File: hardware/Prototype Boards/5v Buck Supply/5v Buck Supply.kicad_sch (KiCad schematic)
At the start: 3 parts, among them J1 BATT, U1 INA180A1IDBVT

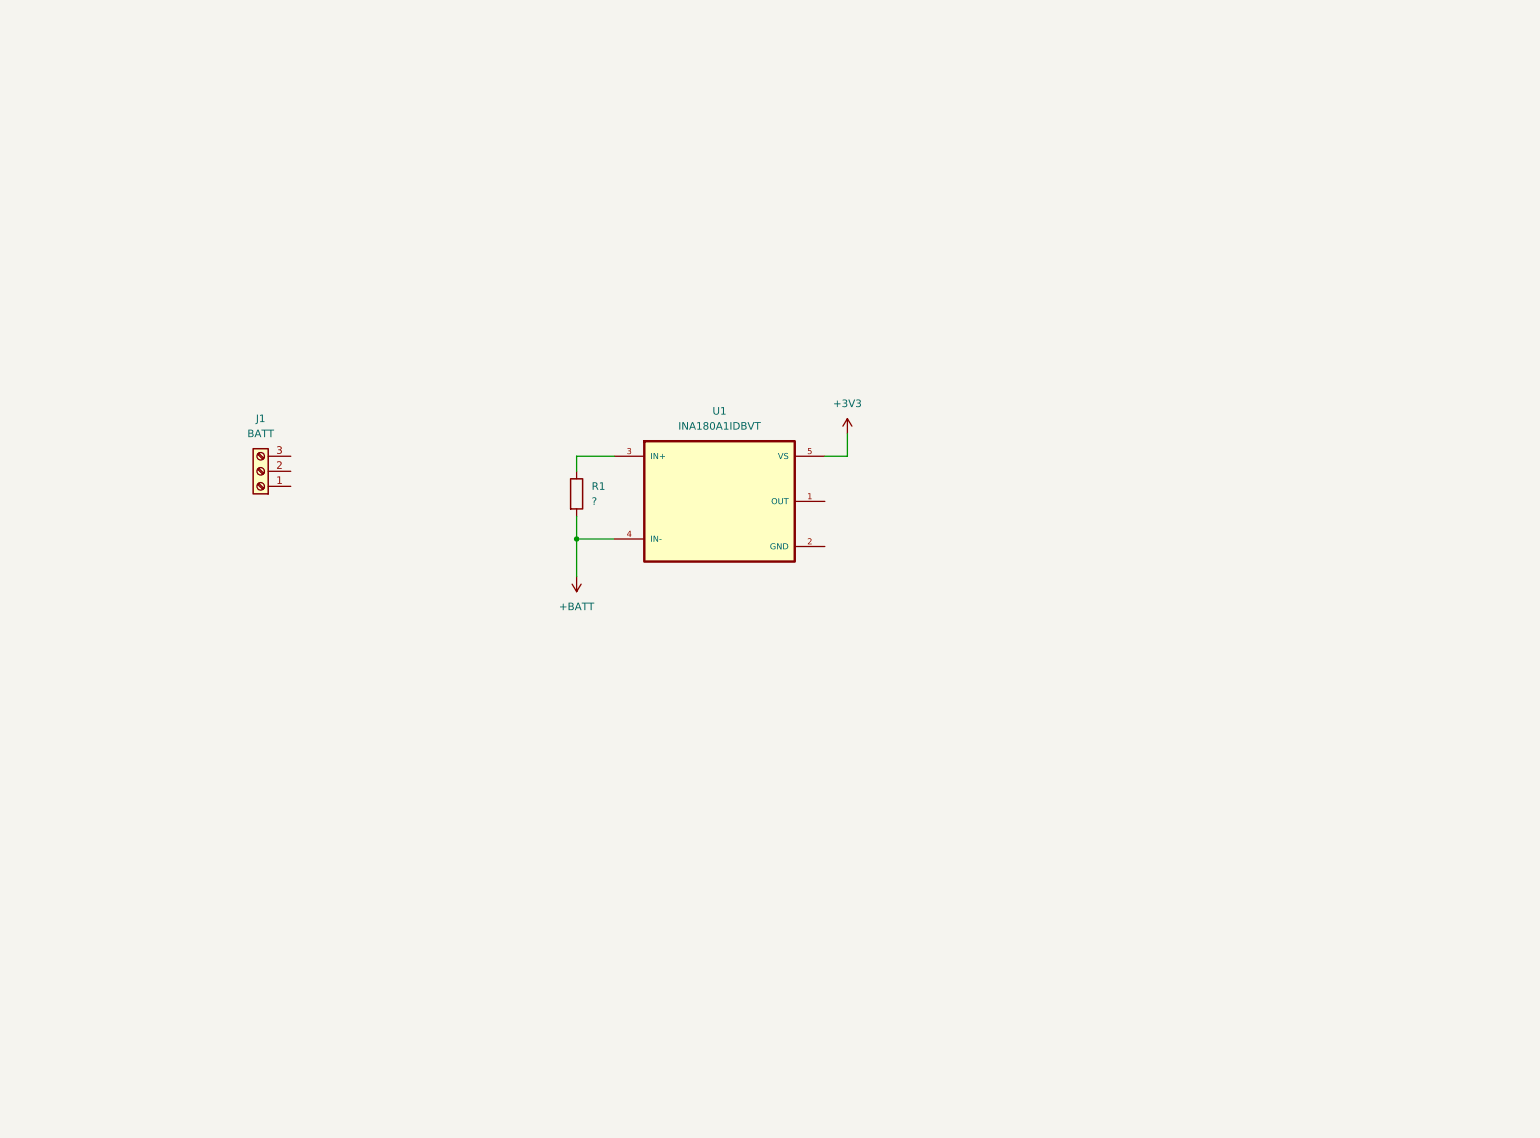
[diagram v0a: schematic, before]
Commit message: sync hardware work
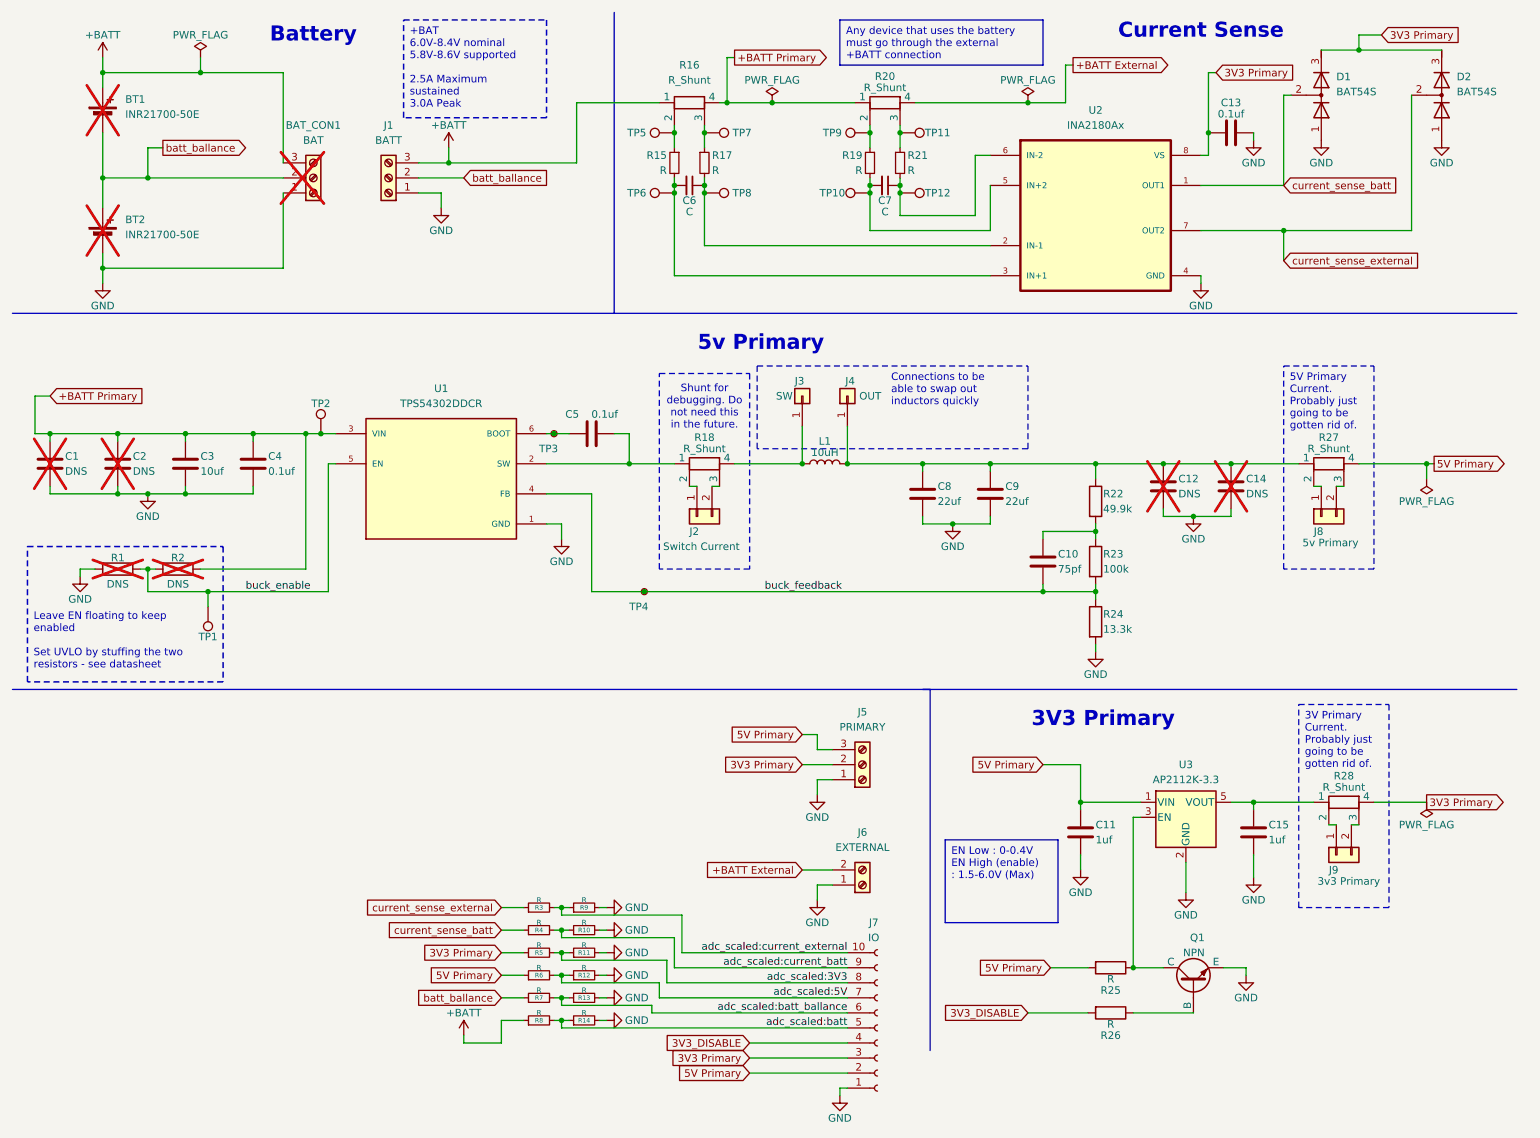
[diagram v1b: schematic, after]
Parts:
- removed U1: INA180A1IDBVT, INA180A1IDBVT:SOT95P280X145-5N, symbol project_symbols:INA180A1IDBVT
- added BAT_CON1: BAT, symbol Connector:Screw_Terminal_01x03
- added BT1, BT2: INR21700-50E, symbol Device:Battery_Cell
- added C1, C2: DNS, Capacitor_SMD:C_1210_3225Metric, symbol Device:C
- added C10: 75pf, Capacitor_SMD:C_0603_1608Metric_Pad1.08x0.95mm_HandSolder, symbol Device:C
- added C11, C15: 1uf, Capacitor_SMD:C_0805_2012Metric, symbol Device:C
- added C12, C14: DNS, Capacitor_SMD:C_1210_3225Metric_Pad1.33x2.70mm_HandSolder, symbol Device:C
- added C13, C4, C5: 0.1uf, Capacitor_SMD:C_0603_1608Metric_Pad1.08x0.95mm_HandSolder, symbol Device:C
- added C3: 10uf, Capacitor_SMD:C_1210_3225Metric, symbol Device:C
- added C6, C7: C, Capacitor_SMD:C_0603_1608Metric_Pad1.08x0.95mm_HandSolder, symbol Device:C_Small
- added C8, C9: 22uf, Capacitor_SMD:C_1210_3225Metric, symbol Device:C
- added D1, D2: BAT54S, Package_TO_SOT_SMD:SOT-23, symbol Device:D_Dual_Series_ACK
- added J2: Switch Current, Connector_PinSocket_2.54mm:PinSocket_1x02_P2.54mm_Vertical, symbol Connector_Generic:Conn_01x02
- added J3: SW, Connector_PinSocket_2.54mm:PinSocket_1x01_P2.54mm_Vertical, symbol Connector_Generic:Conn_01x01
- added J4: OUT, Connector_PinSocket_2.54mm:PinSocket_1x01_P2.54mm_Vertical, symbol Connector_Generic:Conn_01x01
- added J5: PRIMARY, TerminalBlock_TE-Connectivity:TerminalBlock_TE_282834-3_1x03_P2.54mm_Horizontal, symbol Connector:Screw_Terminal_01x03
- added J6: EXTERNAL, TerminalBlock_TE-Connectivity:TerminalBlock_TE_282834-2_1x02_P2.54mm_Horizontal, symbol Connector:Screw_Terminal_01x02
- added J7: IO, Connector_PinHeader_2.54mm:PinHeader_1x10_P2.54mm_Vertical, symbol Connector:Conn_01x10_Socket
- added J8: 5v Primary, Connector_PinSocket_2.54mm:PinSocket_1x02_P2.54mm_Vertical, symbol Connector_Generic:Conn_01x02
- added J9: 3v3 Primary, Connector_PinSocket_2.54mm:PinSocket_1x02_P2.54mm_Vertical, symbol Connector_Generic:Conn_01x02
- added L1: 10uH, footprints:IND_SRU1048-100Y, symbol Device:L
- added Q1: NPN, Package_TO_SOT_SMD:SOT-23, symbol Simulation_SPICE:NPN
- added R10, R11, R12, R13, R14, R15, R17, R19, R21, R3, R4, R5, R6, R7, R8, R9: R, Capacitor_SMD:C_0603_1608Metric_Pad1.08x0.95mm_HandSolder, symbol Device:R_Small
- added R16, R18, R20, R27, R28: R_Shunt, Resistor_SMD:R_0805_2012Metric_Pad1.20x1.40mm_HandSolder, symbol Device:R_Shunt
- added R2: DNS, Resistor_SMD:R_0603_1608Metric_Pad0.98x0.95mm_HandSolder, symbol Device:R
- added R22: 49.9k, Resistor_SMD:R_0603_1608Metric_Pad0.98x0.95mm_HandSolder, symbol Device:R
- added R23: 100k, Resistor_SMD:R_0603_1608Metric_Pad0.98x0.95mm_HandSolder, symbol Device:R
- added R24: 13.3k, Resistor_SMD:R_0603_1608Metric_Pad0.98x0.95mm_HandSolder, symbol Device:R
- added R25, R26: R, Capacitor_SMD:C_0603_1608Metric_Pad1.08x0.95mm_HandSolder, symbol Device:R
- added TP1, TP10, TP11, TP12, TP2, TP5, TP6, TP7, TP8, TP9: TestPoint, footprints:KEYSTONE_5015, symbol Connector:TestPoint
- added TP3, TP4: ~, TestPoint:TestPoint_Pad_D1.5mm, symbol Connector:TestPoint_Small
- added U1: TPS54302DDCR, TPS54302DDCR:SOT95P280X110-6N, symbol project_symbols:TPS54302DDCR
- added U2: INA2180Ax, INA2180A1IDGKR:SOP65P490X110-8N, symbol project_symbols:INA2180A1IDGKR
- added U3: AP2112K-3.3, Package_TO_SOT_SMD:SOT-23-5, symbol Regulator_Linear:AP2112K-3.3
- J1: footprint (none) -> TerminalBlock_TE-Connectivity:TerminalBlock_TE_282834-3_1x03_P2.54mm_Horizontal
- R1: value ? -> DNS; footprint (none) -> Resistor_SMD:R_0603_1608Metric_Pad0.98x0.95mm_HandSolder; now not fitted
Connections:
- net +BATT: now also J1.3 (Pin_3), BAT_CON1.3 (Pin_3), BT1.1 (+), R16.1, R8.1; no longer R1.2
- net GND: now reaches R1.1
- net GND: now also J1.1 (Pin_1), BAT_CON1.1 (Pin_1), BT2.2 (-), C1.2, C11.2, C12.2, C13.2, C14.2, C15.2, C2.2, C3.2, C4.2, C8.2, C9.2, D1.1 (A), D2.1 (A), J5.1 (Pin_1), J6.1 (Pin_1), J7.1 (Pin_1), Q1.3 (E), R10.2, R11.2, R12.2, R13.2, R14.2, R24.2, R9.2, U1.1 (GND), U2.4 (GND), U3.2 (GND)
- net batt_ballance: now reaches J1.2 (Pin_2)
- net batt_ballance: now also BAT_CON1.2 (Pin_2), BT1.2 (-), BT2.1 (+), R7.1
- new net: Q1.1 (C), R25.1, U3.3 (EN)
- new net: Q1.2 (B), R26.1
- new net: C6.2, R15.2, TP6.1, U2.3 (IN+1)
- new net: C7.2, R19.2, TP10.1, U2.5 (IN+2)
- new net: J9.1 (Pin_1), R28.2
- new net: J9.2 (Pin_2), R28.3
- new net: R19.1, R20.2, TP9.1
- new net: R20.3, R21.1, TP11.1
- new net: C5.2, R18.1, U1.2 (SW)
- new net: J2.1 (Pin_1), R18.2
- new net: J2.2 (Pin_2), R18.3
- new net: J3.1 (Pin_1), L1.2, R18.4
- new net: R16.3, R17.1, TP7.1
- new net: C6.1, R17.2, TP8.1, U2.2 (IN-1)
- new net: C7.1, R21.2, TP12.1, U2.6 (IN-2)
- new net: C12.1, C14.1, C8.1, C9.1, J4.1 (Pin_1), L1.1, R22.1, R27.1
- new net: R15.1, R16.2, TP5.1
- new net: C15.1, R28.1, U3.5 (VOUT)
- new net: C5.1, TP3.1, U1.6 (BOOT)
- new net: C10.1, R22.2, R23.1
- new net: J8.1 (Pin_1), R27.2
- new net: J8.2 (Pin_2), R27.3
- new net +BATT External: J6.2 (Pin_2), R20.4
- new net +BATT Primary: C1.1, C2.1, C3.1, C4.1, R16.4, R2.2, R20.1, TP2.1, U1.3 (VIN)
- new net 3V3 Primary: C13.1, D1.3 (K), D2.3 (K), J5.2 (Pin_2), J7.3 (Pin_3), R28.4, R5.1, U2.8 (VS)
- new net 3V3_DISABLE: J7.4 (Pin_4), R26.2
- new net 5V Primary: C11.1, J5.3 (Pin_3), J7.2 (Pin_2), R25.2, R27.4, R6.1, U3.1 (VIN)
- new net adc_scaled:3V3: J7.8 (Pin_8), R11.1, R5.2
- new net adc_scaled:5V: J7.7 (Pin_7), R12.1, R6.2
- new net adc_scaled:batt: J7.5 (Pin_5), R14.1, R8.2
- new net adc_scaled:batt_ballance: J7.6 (Pin_6), R13.1, R7.2
- new net adc_scaled:current_batt: J7.9 (Pin_9), R10.1, R4.2
- new net adc_scaled:current_external: J7.10 (Pin_10), R3.2, R9.1
- new net buck_enable: R1.2, R2.1, TP1.1, U1.5 (EN)
- new net buck_feedback: C10.2, R23.2, R24.1, TP4.1, U1.4 (FB)
- new net current_sense_batt: D1.2 (common), R4.1, U2.1 (OUT1)
- new net current_sense_external: D2.2 (common), R3.1, U2.7 (OUT2)
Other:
- note added: "3V3 Primary"
- note added: "5v Primary"
- note added: "Battery"
- note added: "Current Sense"
- note added: "Shunt for debugging. Do not need this in the future."
- title: (none) -> Prototype Buck Converter
- moved on the sheet: J1
